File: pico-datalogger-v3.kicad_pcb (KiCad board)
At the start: 2 copper layers, 130 x 65 mm, 60 parts, among them IC1 LM66200DRLR, J1 JST-PH2 Bat, J11 Conn_I2C1, J12 Conn_UART_5V, J13 THT_I2C1, J14 THT_I2C0, J17 Disp_THT, J2 Conn_Pico_Left, J3 Conn_Pico_Right, J4 SM06B-GHS-TB_LF_SN, J6 Conn_Display, J9 Conn_I2C0, Q1 AO3401A, Q2 AO3401A, SW1 SW_Push, SW2 SW_Push, SW3 SW_Push, SW4 SW_Push, SW5 SW_Push, U1 74LVC2G74, U2 PCF8523T, U4 XTSD, U5 SCD40_Breakout, U6 AHT20, U7 RFM95W-868S2, Y1 Crystal

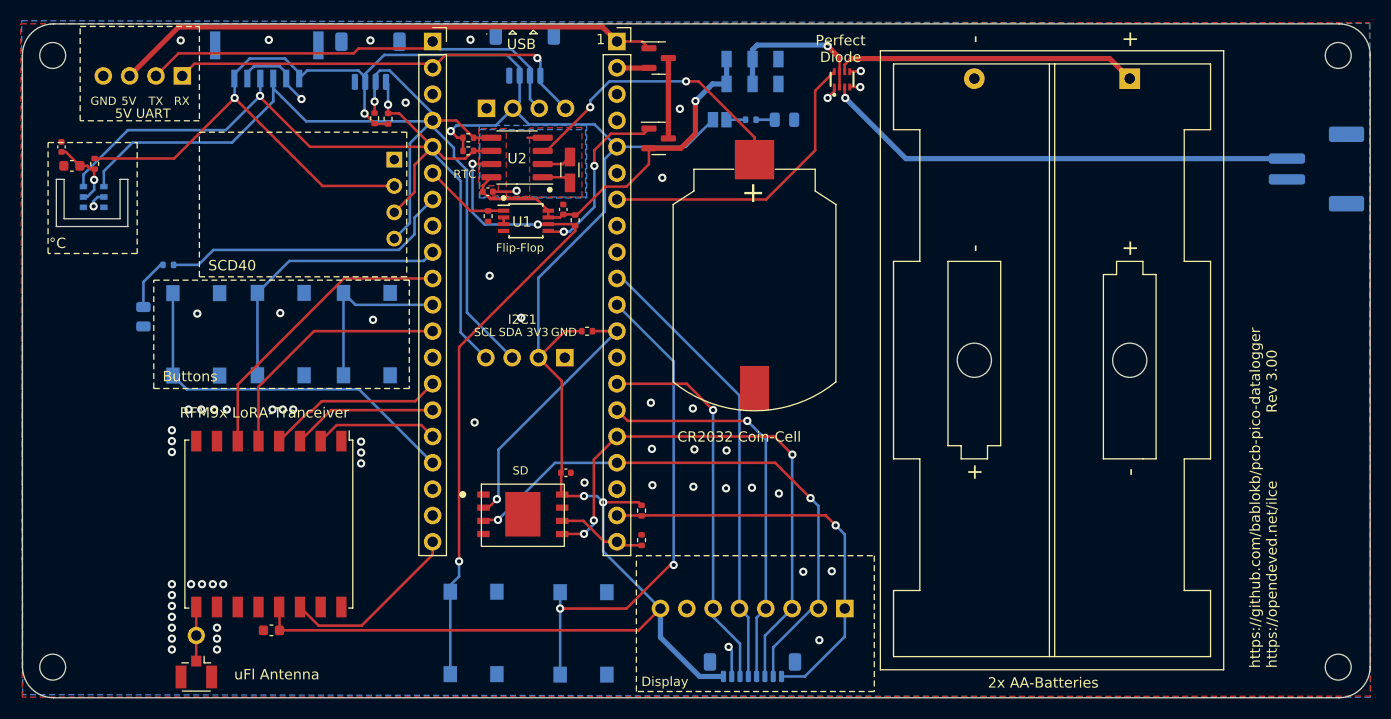
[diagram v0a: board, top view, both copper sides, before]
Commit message: fixes for production files
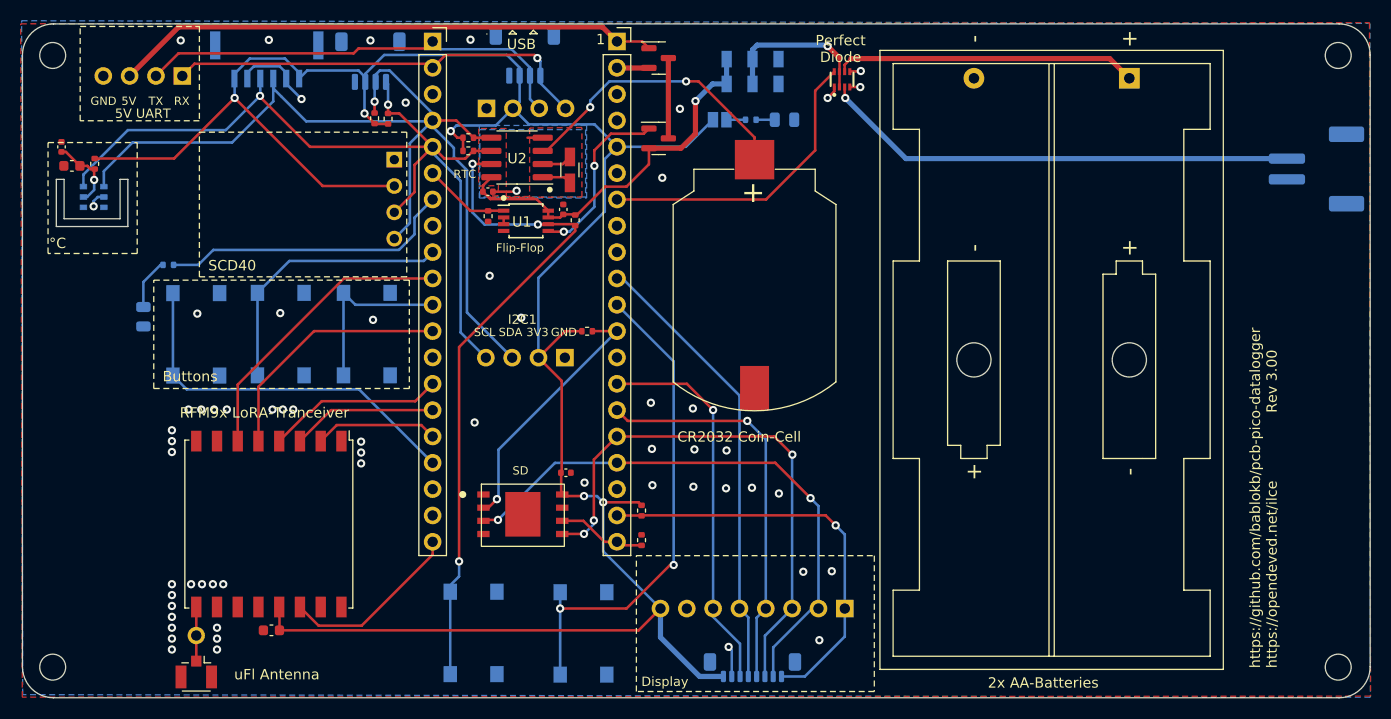
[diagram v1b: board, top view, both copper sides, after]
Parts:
- BT2: footprint Battery:BatteryHolder_Keystone_2462_2xAA -> user:BatteryHolder_Keystone_2462_2xAA
- moved BT2 0.05 mm to (206.8, 105.2)
